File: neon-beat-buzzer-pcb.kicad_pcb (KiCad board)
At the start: 2 copper layers, 78 x 47 mm, 57 parts, among them J1 BATT_CON, J2 SWITCH_CON, J3 BUTTON_CON, J4 USB_C_Receptacle_USB2.0_16P, U1 ESP32-C3-MINI-1, U2 BQ24074RGT, U3 TPS22929D, U4 MCP1700x-330xxTT, U5 TPS610997DRV, U6 USBLC6-2SC6

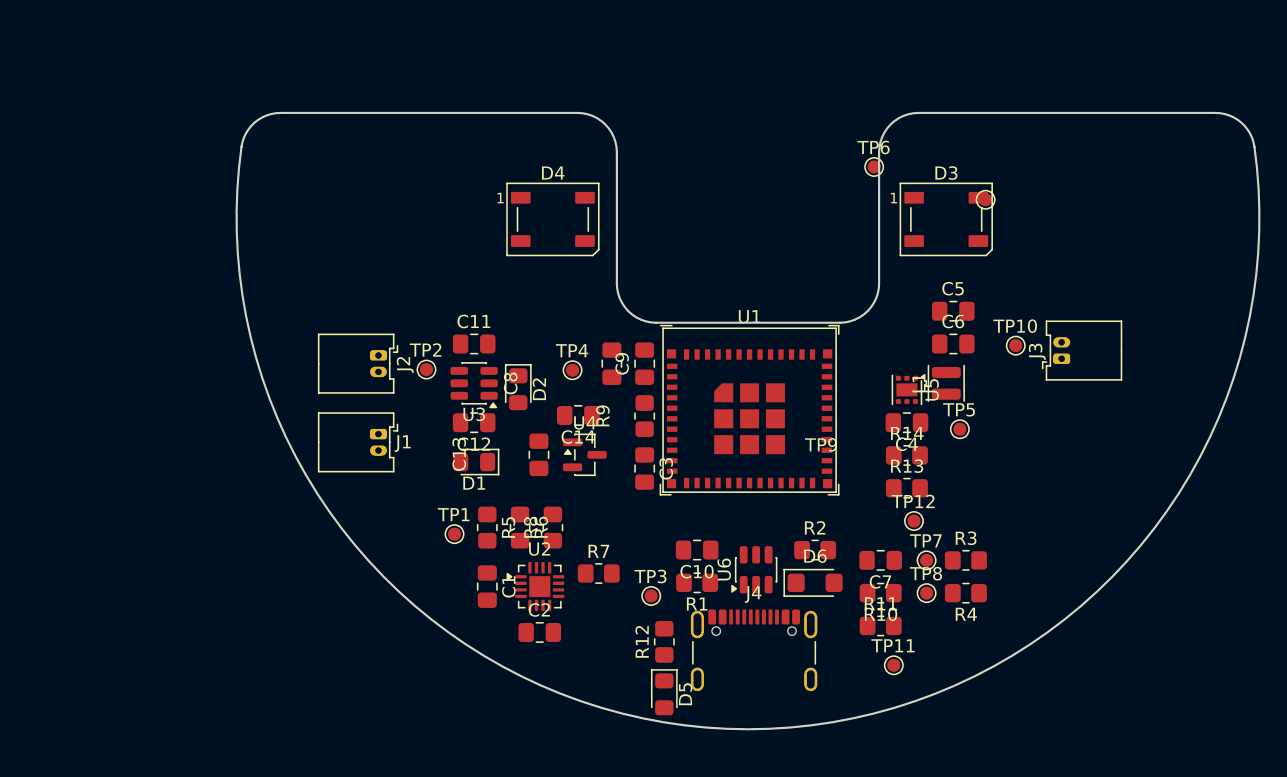
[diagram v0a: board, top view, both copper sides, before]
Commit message: project: partial routing
Signed-off-by: Alexis Lothoré <alexis.lothore@gmail.com>
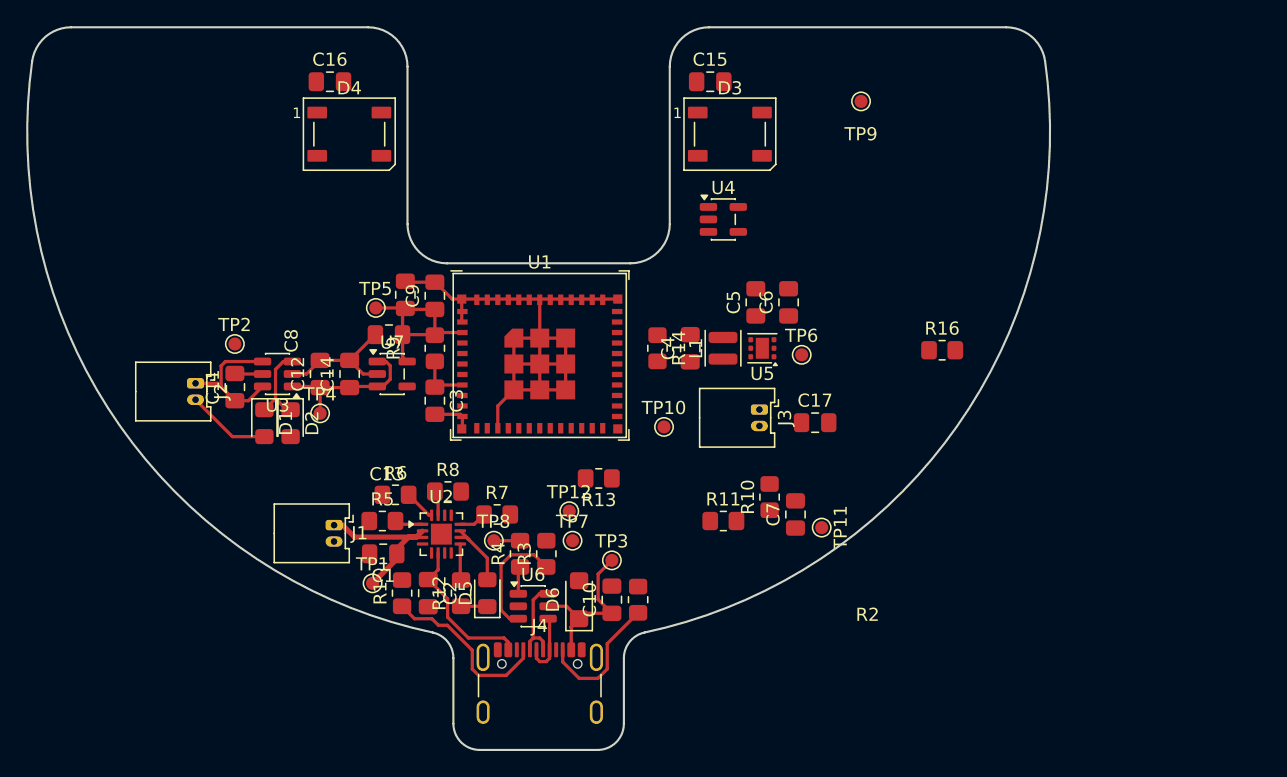
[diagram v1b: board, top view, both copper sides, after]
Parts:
- added C15: 0.1uF, Capacitor_SMD:C_0805_2012Metric_Pad1.18x1.45mm_HandSolder, F.Cu at (147.0, 89.5)
- added C16: 0.1uF, Capacitor_SMD:C_0805_2012Metric_Pad1.18x1.45mm_HandSolder, F.Cu at (118.0, 89.5)
- added C17: 0.1uF, Capacitor_SMD:C_0805_2012Metric_Pad1.18x1.45mm_HandSolder, F.Cu at (155.0, 115.5)
- added R16: 10k, Resistor_SMD:R_0805_2012Metric_Pad1.20x1.40mm_HandSolder, F.Cu at (164.7, 110.0)
- added U7: XC6210B332MR, Package_TO_SOT_SMD:SOT-23-5, F.Cu at (122.8, 111.8)
- U4: value MCP1700x-330xxTT -> 74AHCT1G125; footprint Package_TO_SOT_SMD:SOT-23 -> Package_TO_SOT_SMD:SOT-23-5
- moved TP5 45.5 mm to (121.5, 106.8)
- moved R4 34.1 mm to (132.5, 125.5), turned to 90 degrees
- moved TP8 33.2 mm to (130.5, 124.5)
- moved R3 32.0 mm to (134.5, 125.5), turned to 90 degrees
- moved TP10 27.5 mm to (143.5, 115.8)
- moved TP7 27.0 mm to (136.5, 124.5)
- moved TP12 26.3 mm to (136.2, 122.2)
- moved R13 23.5 mm to (138.5, 119.8), turned to 180 degrees
- moved J3 23.4 mm to (150.8, 114.5), turned to -90 degrees
- moved R1 22.5 mm to (123.5, 128.5), turned to 90 degrees
- moved U4 20.8 mm to (148.0, 100.0)
- moved R14 20.7 mm to (143.0, 109.8), turned to -90 degrees
- moved TP4 19.5 mm to (117.2, 114.8)
- moved C11 18.5 mm to (110.8, 112.8), turned to 90 degrees
- moved D6 18.0 mm to (137.0, 129.0), turned to 90 degrees
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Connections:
- C4 pad 1: /v_3v3 -> /v_sys
- D3 pad 4: /led -> Net-(D3-DIN)
- L1 pad 1: /v_3v3 -> /v_sys
- R13 pad 2: /v_3v3 -> Net-(U5-EN)
- R14 pad 2: /v_3v3 -> /v_sys
- U4 pad 2: /v_3v3 -> /led
- U4 pad 3: /v_ldo -> GND
- U5 pad 6: /v_3v3 -> /v_sys
- U6 pad 1: Net-(J4-D--PadA7) -> Net-(R4-Pad1)
- U6 pad 3: Net-(J4-D+-PadA6) -> Net-(R3-Pad1)
- U6 pad 4: Net-(R3-Pad1) -> Net-(J4-D+-PadA6)
- U6 pad 6: Net-(R4-Pad1) -> Net-(J4-D--PadA7)
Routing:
- net GND: track 0.00 -> 64.0 mm
- net /v_usb: track 0.00 -> 25.6 mm
- net /v_sys: track 0.00 -> 17.8 mm
- net /v_3v3: track 0.00 -> 15.5 mm
- net Net-(J4-CC1): track 0.00 -> 13.5 mm
- net /v_batt_p: track 0.00 -> 12.5 mm
- net /v_ldo: track 0.00 -> 11.9 mm
- net Net-(J4-CC2): track 0.00 -> 10.4 mm
- net Net-(R3-Pad1): track 0.00 -> 9.20 mm
- net Net-(J4-D--PadA7): track 0.00 -> 6.74 mm
- net /switch: track 0.00 -> 6.62 mm
- net Net-(D1-K): track 0.00 -> 6.47 mm
- net Net-(J4-D+-PadA6): track 0.00 -> 4.92 mm
- net Net-(U1-EN/CHIP_PU): track 0.00 -> 4.13 mm
- net /chg: track 0.00 -> 2.78 mm
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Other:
- board size 78 x 47 mm -> 78 x 55.1 mm
